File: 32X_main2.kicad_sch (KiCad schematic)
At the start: 54 parts, among them IC501 SH2 M, IC502 SH2 S, IC503 uPD4502161, IC504 315-5818, IC506 315-5781, IC507 TC511664, IC508 TC511664, IC509 74AC04, IC510 RHSRL33A

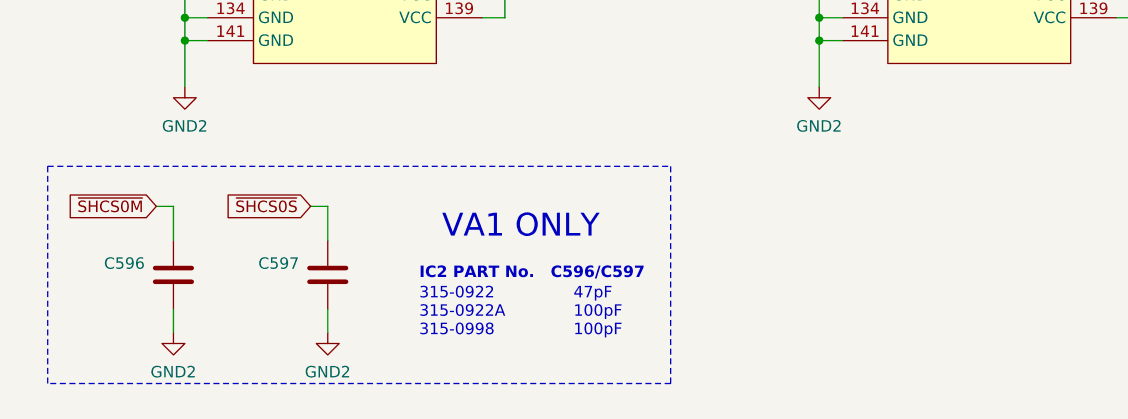
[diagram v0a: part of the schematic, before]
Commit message: General tweaks, add some DigiKey part numbers.
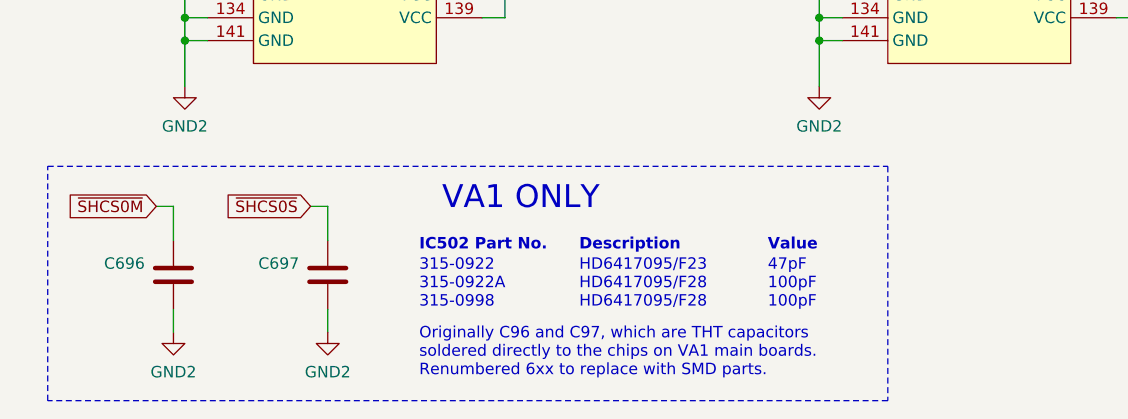
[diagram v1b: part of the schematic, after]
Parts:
- renumbered C596 to C696, C597 to C697
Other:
- note added: "Description"
- note added: "HD6417095/F23 HD6417095/F28 HD6417095/F28"
- note added: "IC502 Part No."
- note added: "Originally C96 and C97, which are THT capacitors soldered directly to the chips on VA1 main boards. Renumbered 6xx to replace with SMD parts."
- note added: "Value"
- note removed: "C596/C597"
- note removed: "IC2 PART No."
